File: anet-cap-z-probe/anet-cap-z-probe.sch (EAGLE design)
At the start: 10 parts, among them X1 12V, X2 EXT-FAN, X3 Z-PROBE, X4 ANET-Z-INPUT

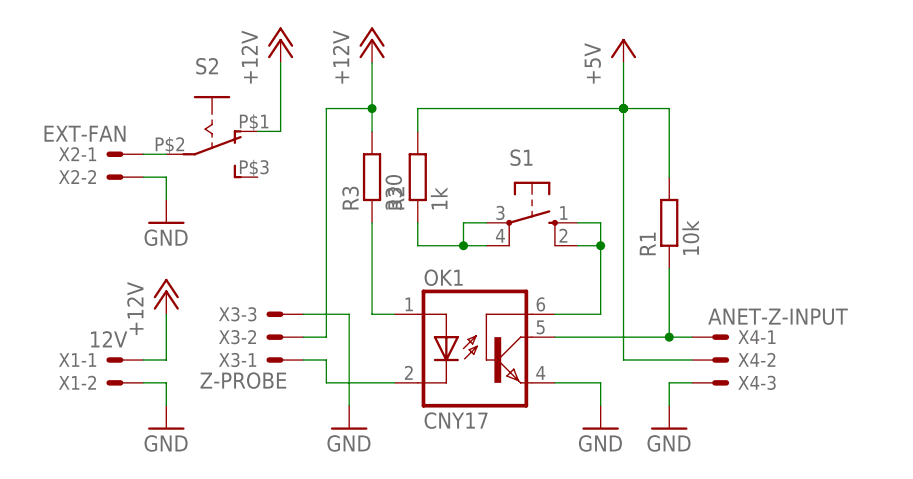
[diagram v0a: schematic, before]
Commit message: new projects
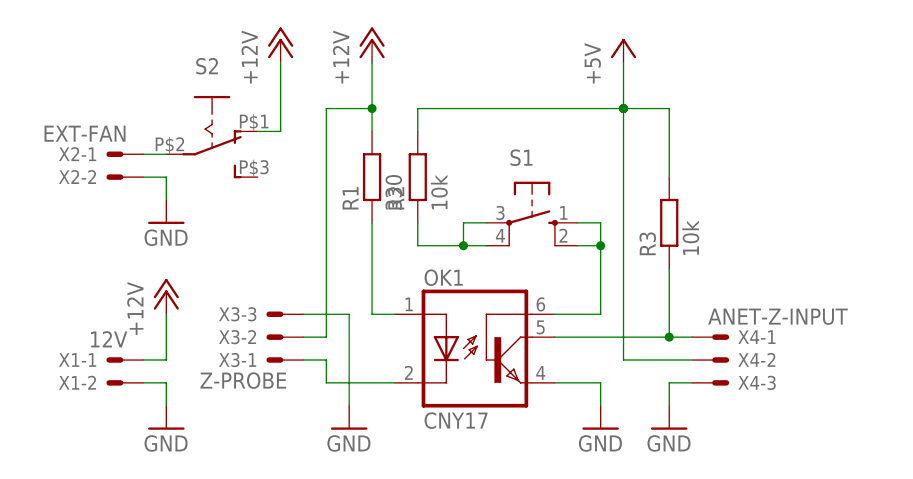
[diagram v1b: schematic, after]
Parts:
- R1: value 10k -> 330; device rcl:R-EU_M0805 -> rcl:R-EU_R0805
- R2: value 1k -> 10k; device rcl:R-EU_M0805 -> rcl:R-EU_R0805
- R3: value 330 -> 10k; device rcl:R-EU_M0805 -> rcl:R-EU_R0805
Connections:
- net +12V: now also R1.2; no longer R3.2
- net +5V: now also R3.2; no longer R1.2
- net N$2: now also R3.1; no longer R1.1
- net N$6: now also R1.1; no longer R3.1
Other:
- moved on the sheet: R1, R3
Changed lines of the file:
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@@
 <part name="GND2" library="supply1" deviceset="GND" device=""/>
 <part name="P+3" library="supply1" deviceset="+12V" device=""/>
-<part name="R1" library="rcl" deviceset="R-EU_" device="M0805" value="10k"/>
-<part name="R2" library="rcl" deviceset="R-EU_" device="M0805" value="1k"/>
-<part name="R3" library="rcl" deviceset="R-EU_" device="M0805" value="330"/>
 <part name="GND3" library="supply1" deviceset="GND" device=""/>
 <part name="GND4" library="supply1" deviceset="GND" device=""/>
@@
 <part name="GND5" library="supply1" deviceset="GND" device=""/>
 <part name="S2" library="_MY_OWN_LIB" deviceset="EG1218" device="THIN"/>
+<part name="R1" library="rcl" deviceset="R-EU_" device="R0805" value="330"/>
+<part name="R2" library="rcl" deviceset="R-EU_" device="R0805" value="10k"/>
+<part name="R3" library="rcl" deviceset="R-EU_" device="R0805" value="10k"/>
 </parts>
 <sheets>
@@
 <instance part="GND2" gate="1" x="22.86" y="96.52"/>
 <instance part="P+3" gate="1" x="35.56" y="116.84"/>
-<instance part="R1" gate="G$1" x="78.74" y="96.52" rot="R90"/>
-<instance part="R2" gate="G$1" x="50.8" y="101.6" rot="R90"/>
-<instance part="R3" gate="G$1" x="45.72" y="101.6" rot="R90"/>
 <instance part="GND3" gate="1" x="78.74" y="73.66"/>
 <instance part="GND4" gate="1" x="71.12" y="73.66"/>
@@
 <instance part="GND5" gate="1" x="43.18" y="73.66"/>
 <instance part="S2" gate="1" x="27.94" y="106.68" rot="R270"/>
+<instance part="R1" gate="G$1" x="45.72" y="101.6" rot="R90"/>
+<instance part="R2" gate="G$1" x="50.8" y="101.6" rot="R90"/>
+<instance part="R3" gate="G$1" x="78.74" y="96.52" rot="R90"/>
 </instances>
 <busses>
@@
 </segment>
 <segment>
-<pinref part="R3" gate="G$1" pin="2"/>
 <pinref part="P+5" gate="1" pin="+12V"/>
 <wire x1="45.72" y1="106.68" x2="45.72" y2="109.22" width="0.1524" layer="91"/>
@@
 <wire x1="40.64" y1="109.22" x2="45.72" y2="109.22" width="0.1524" layer="91"/>
 <junction x="45.72" y="109.22"/>
+<pinref part="R1" gate="G$1" pin="2"/>
 </segment>
 </net>
@@
 <wire x1="73.66" y1="81.28" x2="73.66" y2="109.22" width="0.1524" layer="91"/>
 <pinref part="P+2" gate="1" pin="+5V"/>
-<pinref part="R1" gate="G$1" pin="2"/>
 <wire x1="73.66" y1="109.22" x2="73.66" y2="114.3" width="0.1524" layer="91"/>
 <wire x1="73.66" y1="109.22" x2="78.74" y2="109.22" width="0.1524" layer="91"/>
 <wire x1="78.74" y1="109.22" x2="78.74" y2="101.6" width="0.1524" layer="91"/>
 <junction x="73.66" y="109.22"/>
-<pinref part="R2" gate="G$1" pin="2"/>
 <wire x1="50.8" y1="106.68" x2="50.8" y2="109.22" width="0.1524" layer="91"/>
 <wire x1="50.8" y1="109.22" x2="73.66" y2="109.22" width="0.1524" layer="91"/>
 <junction x="73.66" y="109.22"/>
+<pinref part="R2" gate="G$1" pin="2"/>
+<pinref part="R3" gate="G$1" pin="2"/>
 </segment>
 </net>
@@
 <pinref part="OK1" gate="G$1" pin="COL"/>
 <wire x1="81.28" y1="83.82" x2="78.74" y2="83.82" width="0.1524" layer="91"/>
-<pinref part="R1" gate="G$1" pin="1"/>
 <wire x1="78.74" y1="83.82" x2="66.04" y2="83.82" width="0.1524" layer="91"/>
 <wire x1="78.74" y1="91.44" x2="78.74" y2="83.82" width="0.1524" layer="91"/>
 <junction x="78.74" y="83.82"/>
+<pinref part="R3" gate="G$1" pin="1"/>
 </segment>
 </net>
 <net name="N$4" class="0">
 <segment>
-<pinref part="R2" gate="G$1" pin="1"/>
 <wire x1="50.8" y1="96.52" x2="50.8" y2="93.98" width="0.1524" layer="91"/>
 <pinref part="S1" gate="1" pin="P1"/>
@@
 <wire x1="55.88" y1="96.52" x2="55.88" y2="93.98" width="0.1524" layer="91"/>
 <junction x="55.88" y="93.98"/>
+<pinref part="R2" gate="G$1" pin="1"/>
 </segment>
 </net>
@@
 <net name="N$6" class="0">
 <segment>
-<pinref part="R3" gate="G$1" pin="1"/>
 <wire x1="45.72" y1="96.52" x2="45.72" y2="86.36" width="0.1524" layer="91"/>
 <pinref part="OK1" gate="G$1" pin="A"/>
 <wire x1="45.72" y1="86.36" x2="48.26" y2="86.36" width="0.1524" layer="91"/>
+<pinref part="R1" gate="G$1" pin="1"/>
 </segment>
 </net>
